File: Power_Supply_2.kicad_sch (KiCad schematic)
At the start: 12 parts

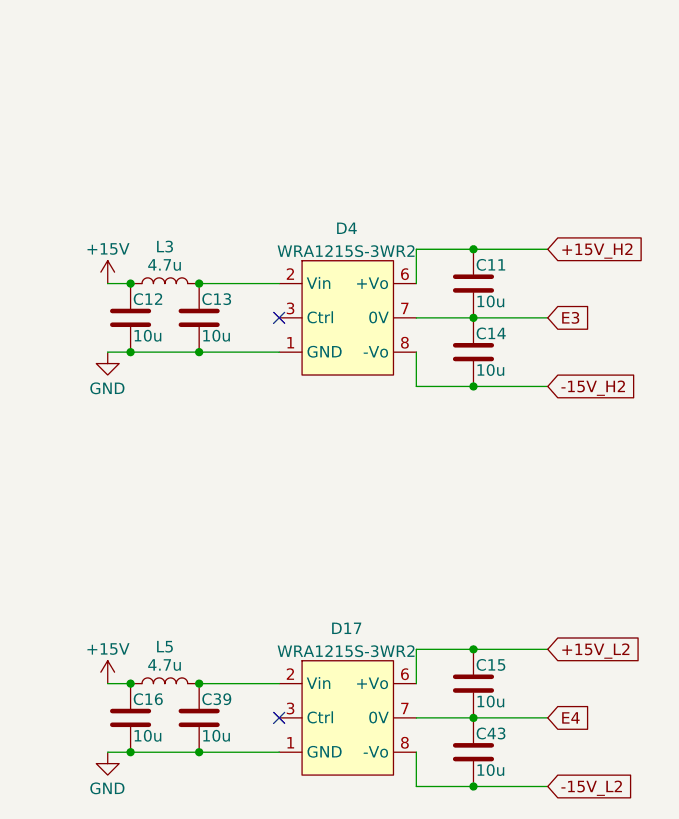
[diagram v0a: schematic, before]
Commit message: VER2.2: все изменения в списке изменений
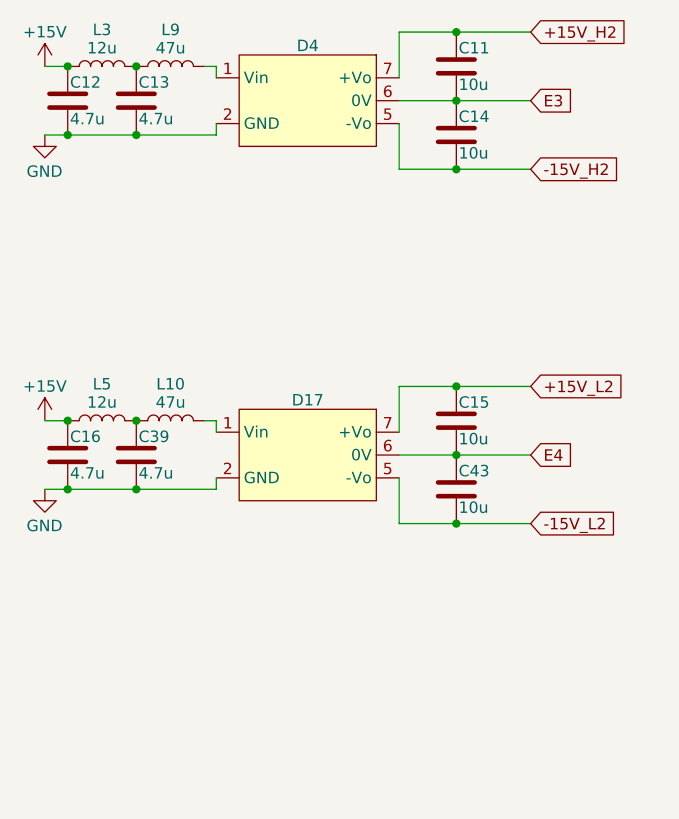
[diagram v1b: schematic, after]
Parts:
- removed D17, D4: WRA1215S-3WR2, Mornsun:WRA_S-3WR2, symbol Morsun:WRA1215S-3WR2
- added D17, D4: ~, DCDC_My:QA, symbol DCDC_My:QA1
- added L10, L9: 47u, Inductor_SMD:L_1812_4532Metric_Pad1.30x3.40mm_HandSolder, symbol Device:L
- C12, C13, C16, C39: value 10u -> 4.7u; footprint Capacitor_SMD:C_1210_3225Metric_Pad1.33x2.70mm_HandSolder -> Capacitor_SMD:C_1206_3216Metric_Pad1.33x1.80mm_HandSolder
- L3, L5: value 4.7u -> 12u; footprint Inductor_SMD:L_1812_4532Metric_Pad1.30x3.40mm_HandSolder -> Inductor_SMD:L_1210_3225Metric_Pad1.42x2.65mm_HandSolder; Product Name (none) -> LQH32MN120J23L
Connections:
- net +15V_H2: now also D4.7 (+Vo)
- net +15V_L2: now also D17.7 (+Vo)
- net -15V_H2: now also D4.5 (-Vo)
- net -15V_L2: now also D17.5 (-Vo)
- net E3: now also D4.6 (0V)
- net E4: now also D17.6 (0V)
- net GND: now also D17.2 (GND), D4.2 (GND)
- net at C39.1, L5.2: now also L10.1
- net at C13.1, L3.2: now also L9.1
- new net: D17.1 (Vin), L10.2
- new net: D4.1 (Vin), L9.2
- no-connect marks 2 -> 0
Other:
- moved on the sheet: C11, C12, C13, C14, C15, C16, C39, C43, L3, L5
